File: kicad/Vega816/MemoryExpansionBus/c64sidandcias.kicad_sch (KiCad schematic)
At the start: 9 parts, among them J62 IRQ_OUT, J63 Device Select, J64 A/D Bus, J72 $80 (32B), J76 $00 (16B), J77 $40 (16B)

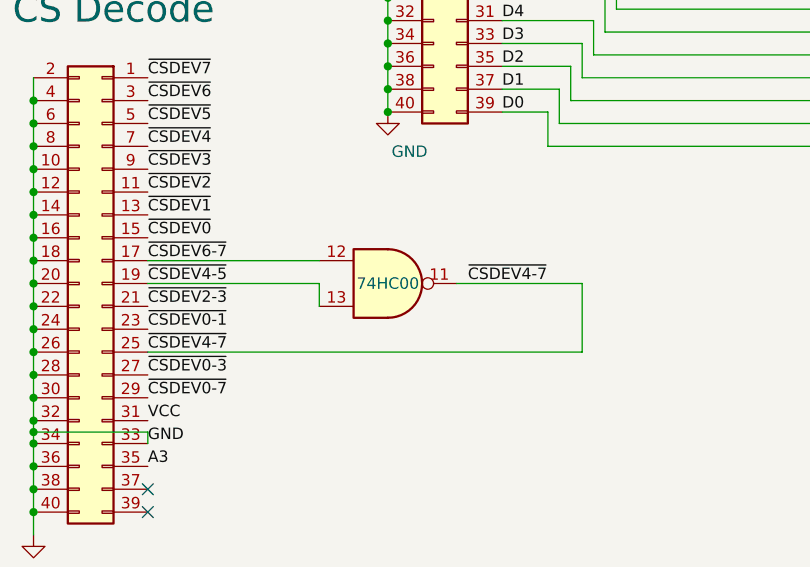
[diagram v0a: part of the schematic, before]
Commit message: Big push, Sysctl, DMA Reg
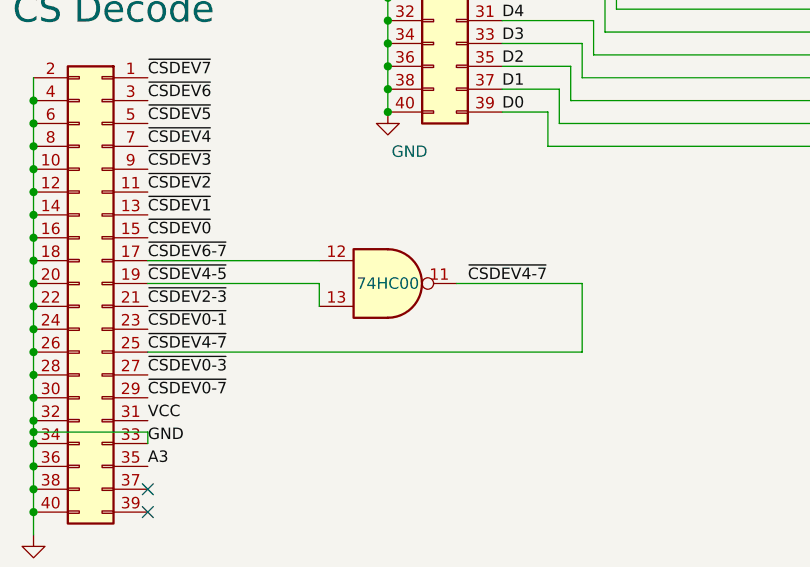
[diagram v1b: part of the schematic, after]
